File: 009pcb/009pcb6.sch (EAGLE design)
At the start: 27 parts

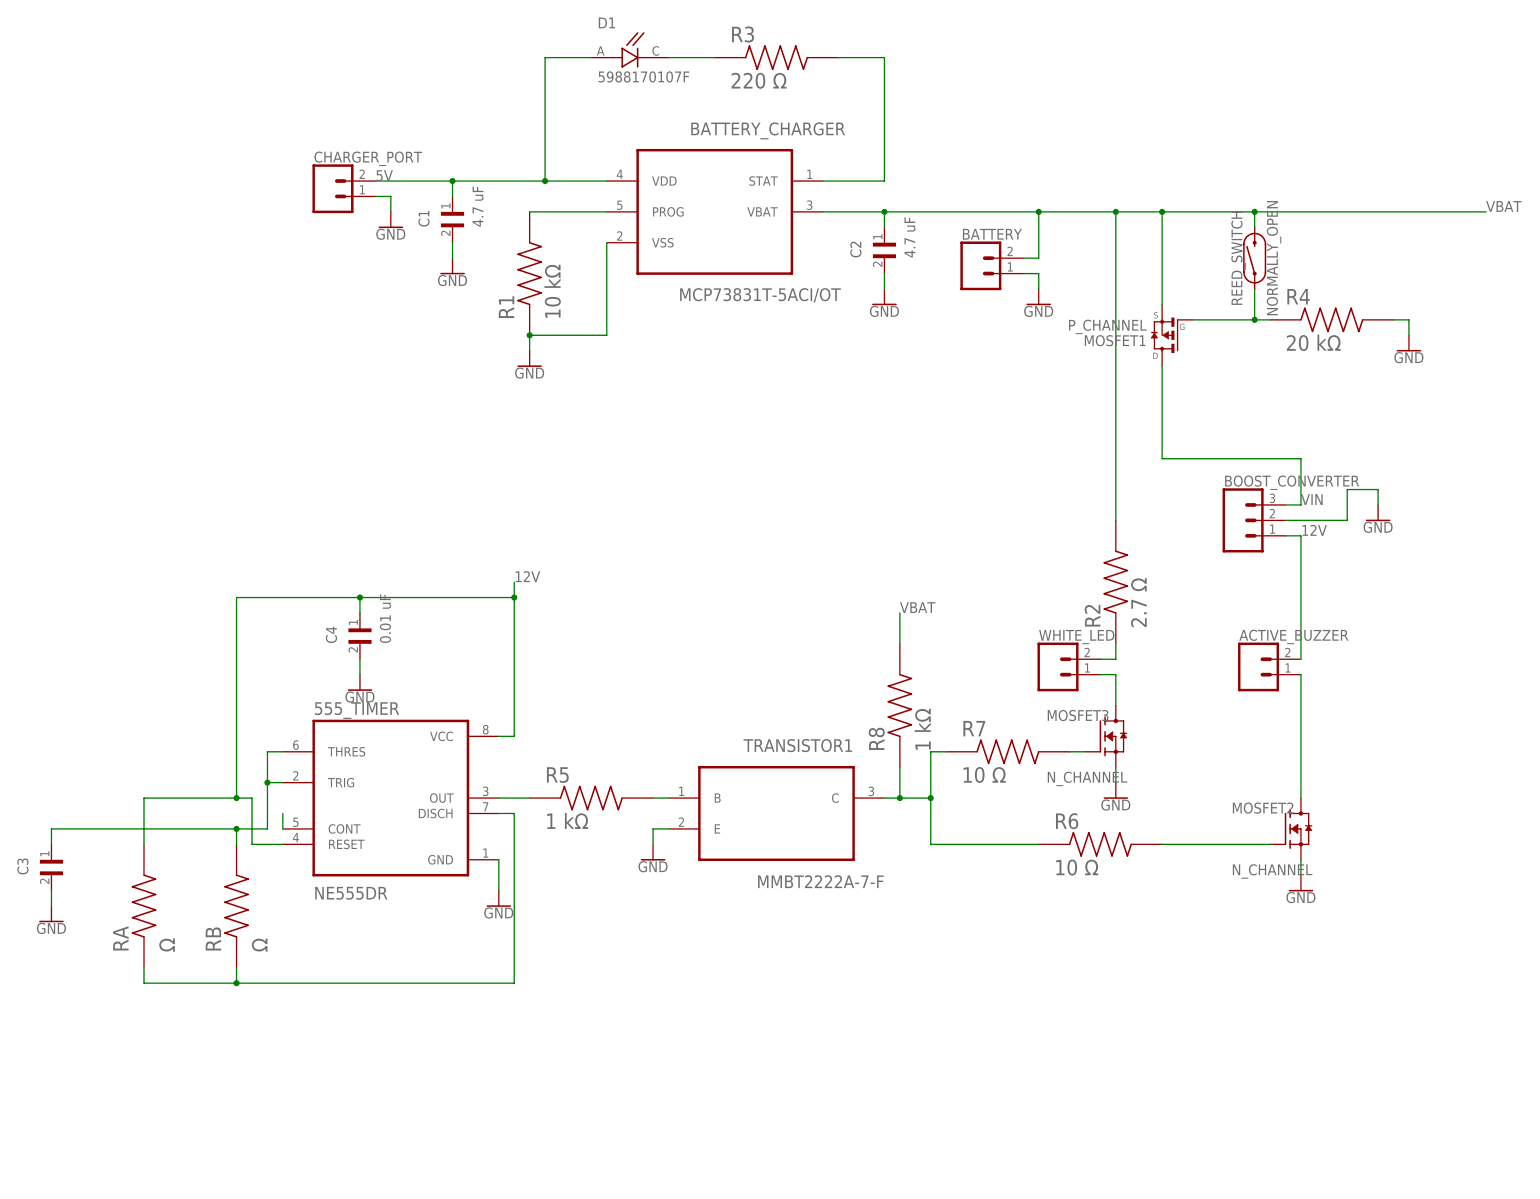
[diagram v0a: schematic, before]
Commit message: 009pcb6.brd
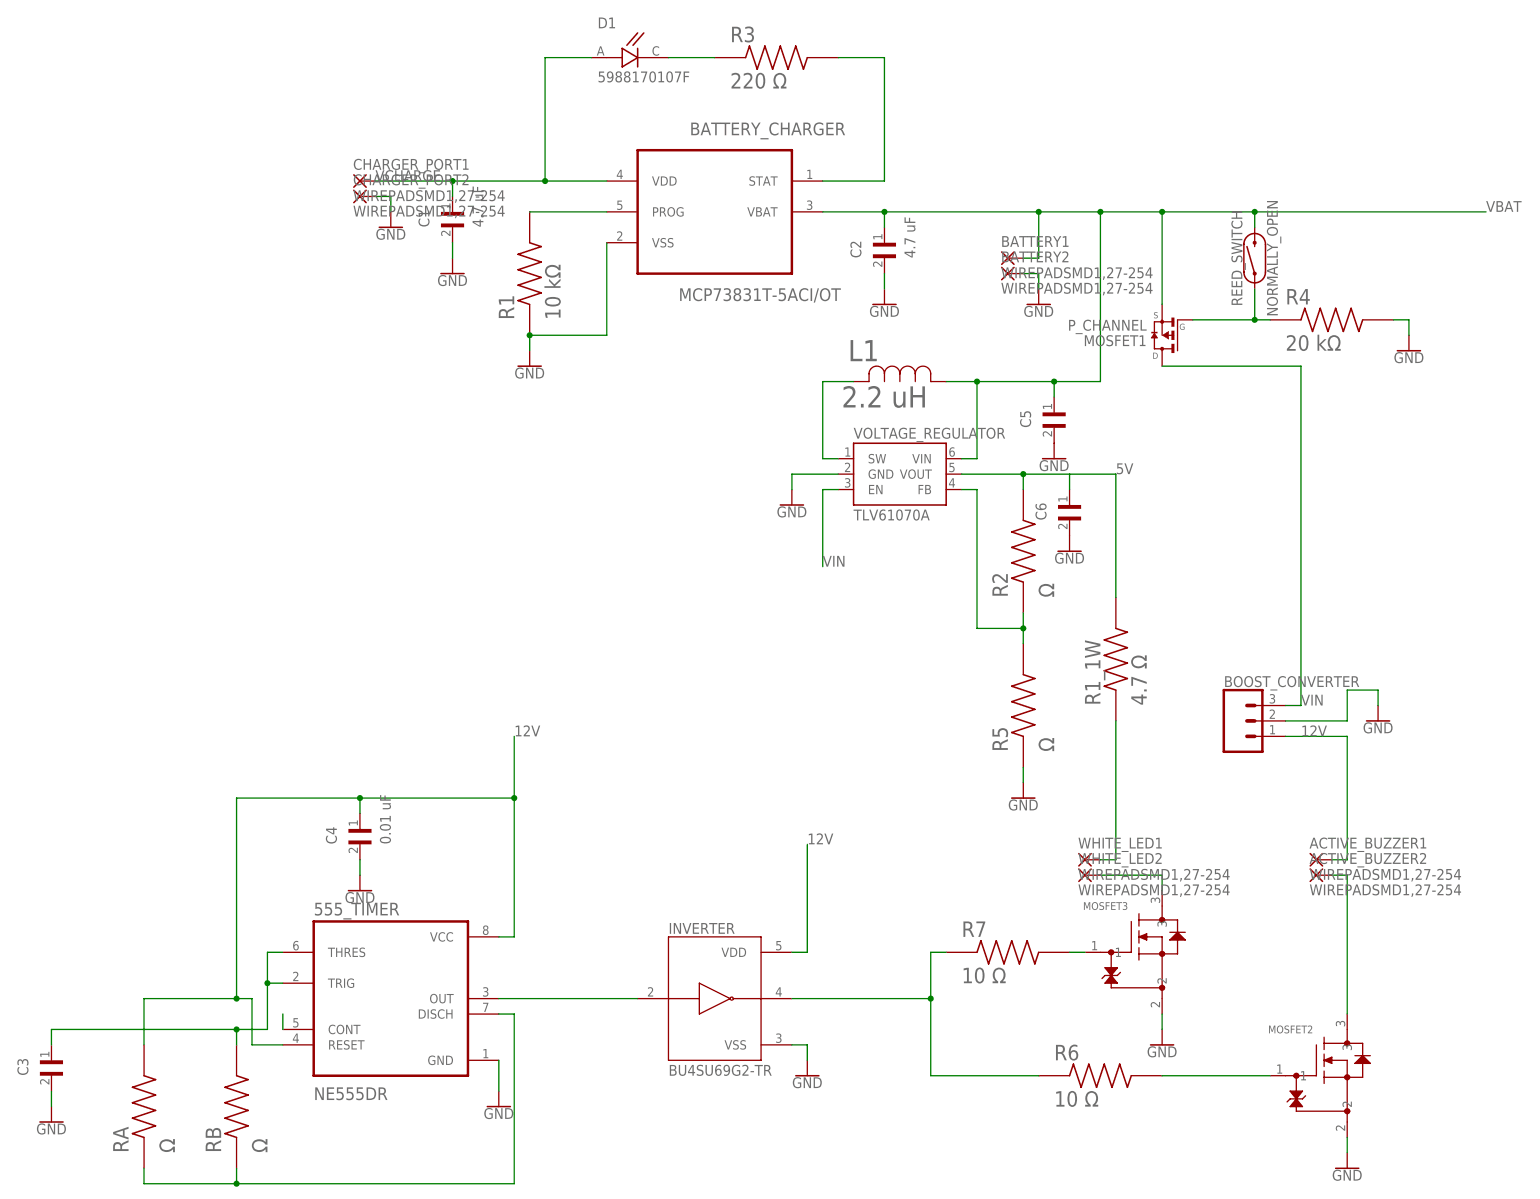
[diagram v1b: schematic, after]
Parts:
- removed ACTIVE_BUZZER, BATTERY, CHARGER_PORT, WHITE_LED: (no value), SparkFun-Connectors:CONN_02
- removed R8: 1 kΩ, RC0805JR-0720KL:RC0805JR-0720KL
- removed TRANSISTOR1: MMBT2222A-7-F, MMBT2222A-7-F:MMBT2222A-7-F
- added ACTIVE_BUZZER1, ACTIVE_BUZZER2, BATTERY1, BATTERY2, CHARGER_PORT1, CHARGER_PORT2, WHITE_LED1, WHITE_LED2: WIREPADSMD1,27-254, wirepad:WIREPADSMD1,27-254
- added C5, C6: GRT21BR61H475ME13L, GRT21BR61H475ME13L:GRT21BR61H475ME13L
- added INVERTER: BU4SU69G2-TR, BU4SU69G2-TR:BU4SU69G2-TR
- added L1: 2.2 uH, 74438357022:74438357022
- added R1_1W: 4.7 Ω, RC2512FK-074R7L:RC2512FK-074R7L
- added VOLTAGE_REGULATOR: TLV61070A, TLV61070A:TLV61070ASOT-23
- MOSFET2, MOSFET3: value N_CHANNEL -> SSM3K335R; device AO3400A:AO3400A -> SSM3K335R:SSM3K335R
- R2: value 2.7 Ω -> Ω; device RCS08052R70FKEA:RCS08052R70FKEA -> RC0805JR-0720KL:RC0805JR-0720KL
- R5: value 1 kΩ -> Ω
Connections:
- removed net N$16: R2.1, WHITE_LED.2
- new net N$10: L1.2, VOLTAGE_REGULATOR.SW
- new net N$7: R1_1W.1, WHITE_LED1.P
- new net VBAT1: C6.1
- new net VCHARGE: BATTERY_CHARGER.VDD, C1.1, CHARGER_PORT1.P, D1.A
- net 12V: now also ACTIVE_BUZZER1.P, INVERTER.VDD; no longer ACTIVE_BUZZER.2
- net 5V: now also R1_1W.2, R2.2, VOLTAGE_REGULATOR.VOUT; no longer BATTERY_CHARGER.VDD, C1.1, CHARGER_PORT.2, D1.A
- net GND: now also BATTERY2.P, C5.2, C6.2, CHARGER_PORT2.P, INVERTER.VSS, MOSFET2.2, MOSFET3.2, R5.1, VOLTAGE_REGULATOR.GND; no longer BATTERY.1, CHARGER_PORT.1, MOSFET2.S, MOSFET3.S, TRANSISTOR1.E
- net N$11: now also INVERTER.A; no longer R5.1
- net N$12: now also R2.1, VOLTAGE_REGULATOR.FB; no longer TRANSISTOR1.B
- net N$13: now also INVERTER.Y; no longer R8.1, TRANSISTOR1.C
- net N$14: now also MOSFET3.1; no longer MOSFET3.G
- net N$15: now also MOSFET3.3, WHITE_LED2.P; no longer MOSFET3.D, WHITE_LED.1
- net N$18: now also MOSFET2.1; no longer MOSFET2.G
- net N$19: now also ACTIVE_BUZZER2.P, MOSFET2.3; no longer ACTIVE_BUZZER.1, MOSFET2.D
- net VBAT: now also BATTERY1.P, C5.1, L1.1, VOLTAGE_REGULATOR.VIN; no longer BATTERY.2, R2.2, R8.2
- net VIN: now also VOLTAGE_REGULATOR.EN
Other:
- moved on the sheet: 555_TIMER, BOOST_CONVERTER, C3, C4, R2, R5, R6, R7, RA, RB
